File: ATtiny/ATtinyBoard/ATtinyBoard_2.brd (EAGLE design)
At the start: 100 x 80 mm, 19 parts, among them IC2 TINY13-20SU

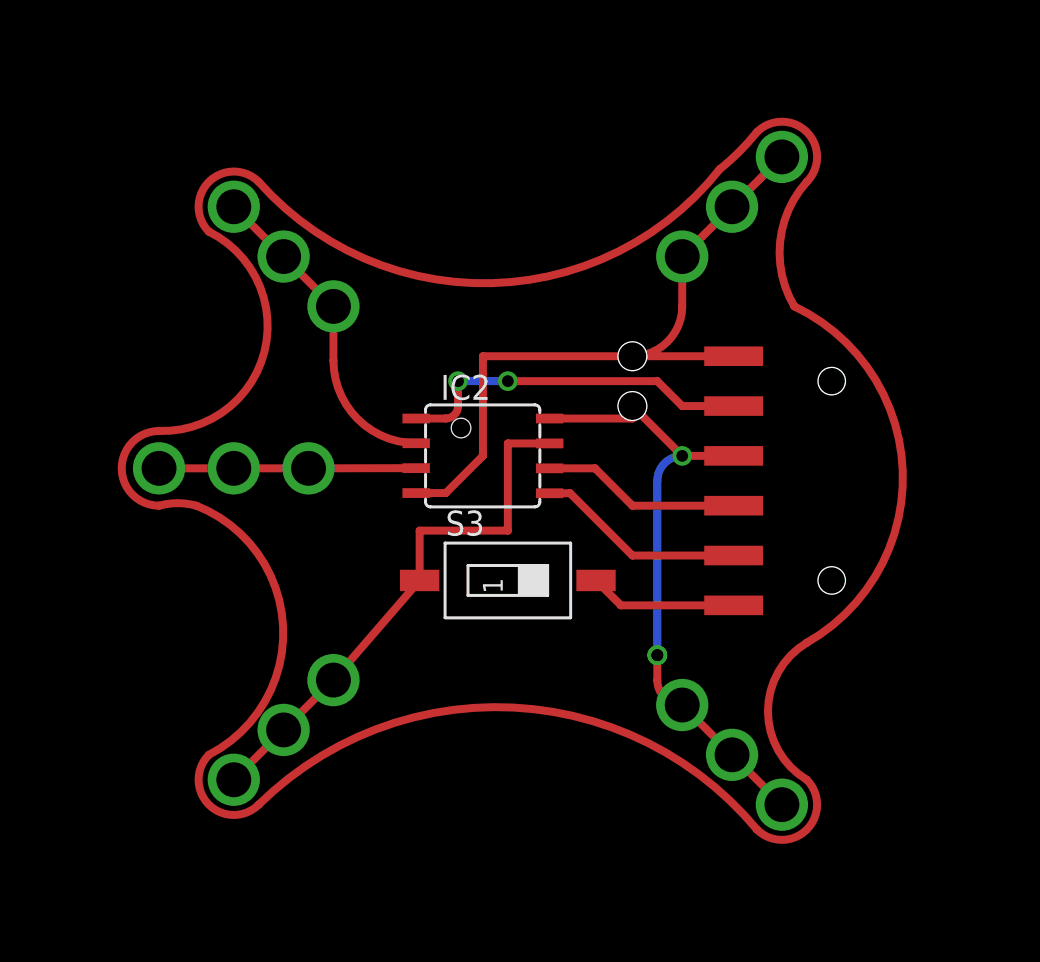
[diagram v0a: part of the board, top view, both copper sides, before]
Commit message: folder re-ordering
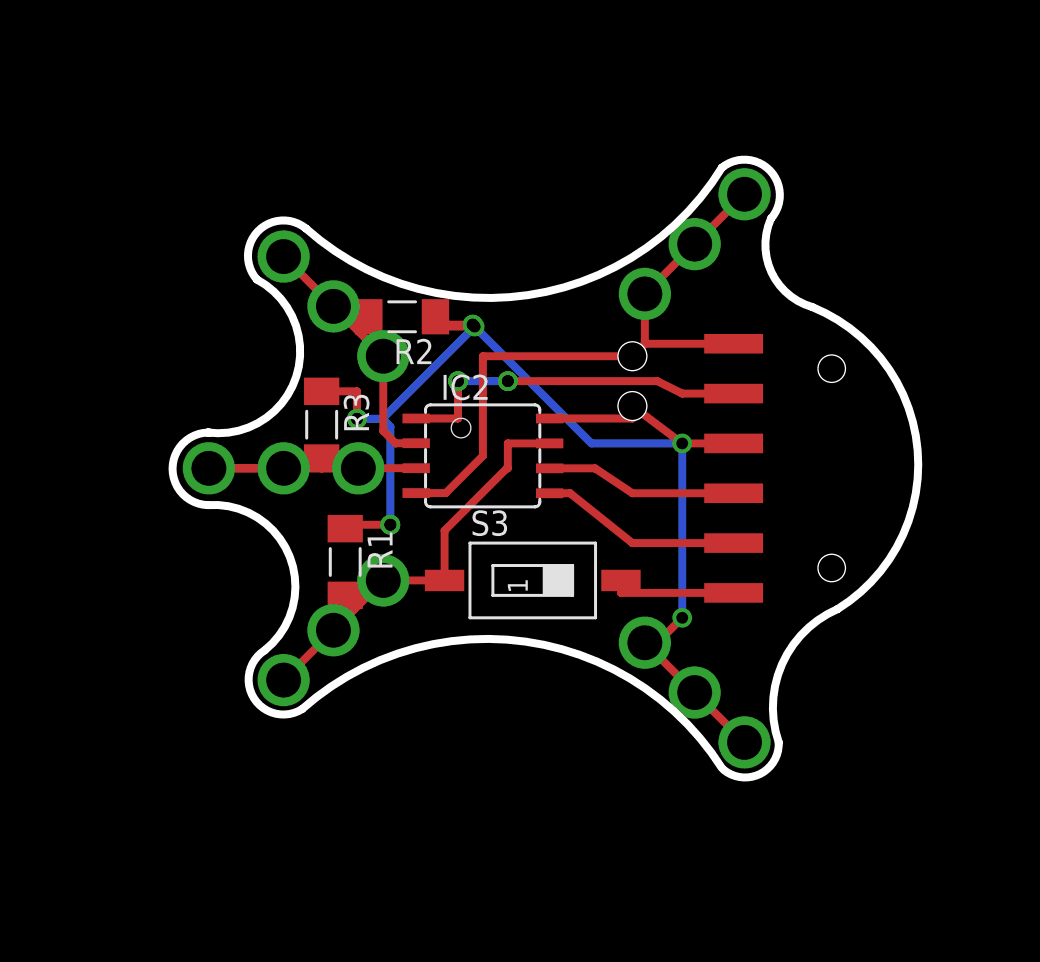
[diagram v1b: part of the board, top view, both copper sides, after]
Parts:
- added R1, R2, R3: (no value), resistor:M1406
- moved H13 12.7 mm to (40.6, 35.6)
- moved H11 10.8 mm to (40.6, 47.0)
- moved H9 10.2 mm to (39.4, 41.3)
- moved H15 9.88 mm to (54.0, 50.2)
- moved H7 3.70 mm to (59.1, 27.3)
- moved H5 3.70 mm to (54.0, 32.4)
- moved H6 3.70 mm to (56.5, 29.8)
- moved H1 2.54 mm to (38.1, 33.0)
- moved H12 2.54 mm to (35.6, 30.5)
- moved H8 1.27 mm to (31.8, 41.3)
- moved H3 1.27 mm to (35.6, 41.3)
- moved S3 1.27 mm to (48.3, 35.6)
- moved H14 0.90 mm to (59.1, 55.2)
- moved H4 0.90 mm to (56.5, 52.7)
- moved ISP/FTDI-CONNECTOR 0.63 mm to (63.5, 41.3)
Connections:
- removed net N$2: H3.P$1, H8.P$1, H9.P$1, IC2.3
- removed net N$6: H10.P$1, H11.P$1, H2.P$1, IC2.2
- removed net N$7: H5.P$1, H6.P$1, H7.P$1, IC2.8, ISP/FTDI-CONNECTOR.4, JP2.2
- removed net N$8: H1.P$1, H12.P$1, H13.P$1, IC2.7, S3.1
- new net PB2: H1.P$1, H12.P$1, H13.P$1, IC2.7, R1.2, S3.1
- new net PB3: H10.P$1, H11.P$1, H2.P$1, IC2.2, R2.2
- new net PB4: H3.P$1, H8.P$1, H9.P$1, IC2.3, R3.2
- new net VCC: H5.P$1, H6.P$1, H7.P$1, IC2.8, ISP/FTDI-CONNECTOR.4, JP2.2, R1.1, R2.1, R3.1
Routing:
- net N$10: track 125.4 -> 0.00 mm
- net VCC: track 0.00 -> 65.8 mm, vias 0 -> 6
- net N$7: track 32.0 -> 0.00 mm, vias 2 -> 0
- net N$8: track 27.5 -> 0.00 mm
- net PB2: track 0.00 -> 22.0 mm
- net PB4: track 0.00 -> 18.7 mm
- net N$6: track 15.9 -> 0.00 mm
- net PB3: track 0.00 -> 14.2 mm
- net N$2: track 13.1 -> 0.00 mm
- net GND: track 42.5 -> 32.0 mm
- net N$5: track 7.54 -> 6.38 mm
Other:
- outline, holes or cut-outs redrawn
